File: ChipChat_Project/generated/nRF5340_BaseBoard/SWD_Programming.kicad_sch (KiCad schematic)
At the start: 1 part, among them J1 Connector_Generic:Conn_02x05_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

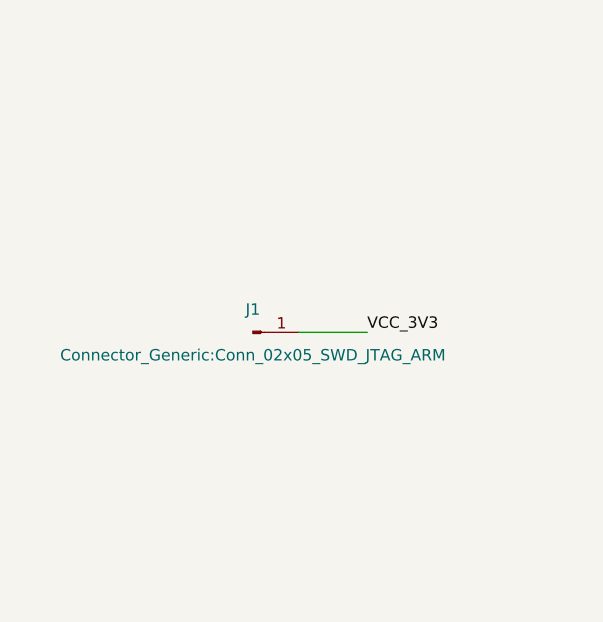
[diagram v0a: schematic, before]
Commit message: 💾 snapshot 2026-03-23_13-16-53
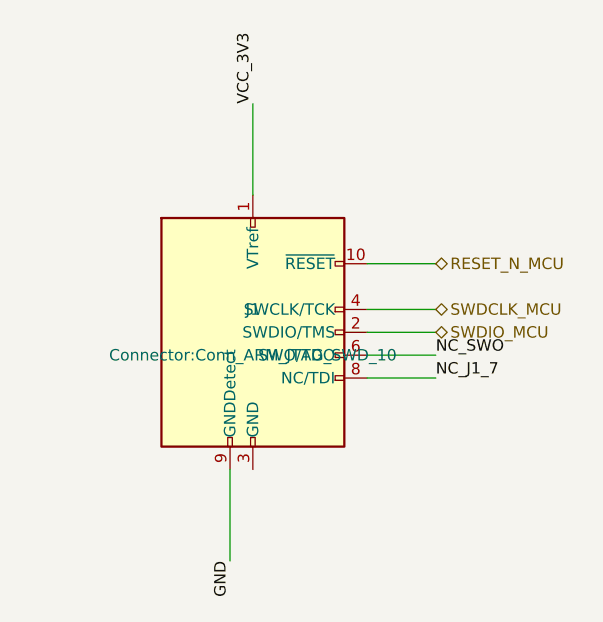
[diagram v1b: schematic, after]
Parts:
- removed J1: Connector_Generic:Conn_02x05_SWD_JTAG_ARM, symbol Conn_01x01_Pin
- added J1: Connector:Conn_ARM_JTAG_SWD_10, symbol Conn_ARM_JTAG_SWD_10
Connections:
- net VCC_3V3: now also J1.1 (VTref)
- new net: J1.3 (GND), J1.5 (GND)
- new net GND: J1.9 (GNDDetect)
- new net NC_J1_7: J1.8 (NC/TDI)
- new net NC_SWO: J1.6 (SWO/TDO)
- new net RESET_N_MCU: J1.10 (~{RESET})
- new net SWDCLK_MCU: J1.4 (SWCLK/TCK)
- new net SWDIO_MCU: J1.2 (SWDIO/TMS)
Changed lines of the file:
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@@
 	(paper "A4")
 	(symbol
-		(lib_id "Conn_01x01_Pin")
+		(lib_id "Conn_ARM_JTAG_SWD_10")
 		(at 200.0 100.0 0)
 		(unit 1)
@@
 			)
 		)
-		(property "Value" "Connector_Generic:Conn_02x05_SWD_JTAG_ARM"
+		(property "Value" "Connector:Conn_ARM_JTAG_SWD_10"
 			(at 200.0 102.54 0)
 			(effects
@@
 		(pin "1"
 		)
+		(pin "2"
+		)
+		(pin "3"
+		)
+		(pin "4"
+		)
+		(pin "5"
+		)
+		(pin "6"
+		)
+		(pin "7"
+		)
+		(pin "8"
+		)
+		(pin "9"
+		)
+		(pin "10"
+		)
 	)
 	(wire
 		(pts
-			(xy 205.08 100.0) (xy 212.7 100.0)
+			(xy 200.0 84.76) (xy 200.0 74.6)
 		)
 		(stroke
@@
 	)
 	(label "VCC_3V3"
-		(at 212.7 100.0 0)
+		(at 200.0 74.6 90)
 		(effects
 			(font
@@
 		)
 	)
+	(wire
+		(pts
+			(xy 212.7 100.0) (xy 220.32 100.0)
+		)
+		(stroke
+			(width 0)
+			(type default)
+		)
+	)
+	(hierarchical_label "SWDIO_MCU"
+		(shape bidirectional)
+		(at 220.32 100.0 0)
+		(effects
+			(font
+				(size 1.27 1.27)
+			)
+			(justify left)
+		)
+	)
+	(wire
+		(pts
+			(xy 197.46 115.24) (xy 197.46 125.4)
+		)
+		(stroke
+			(width 0)
+			(type default)
+		)
+	)
+	(label "GND"
+		(at 197.46 125.4 90)
+		(effects
+			(font
+				(size 1.27 1.27)
+			)
+			(justify right bottom)
+		)
+	)
+	(wire
+		(pts
+			(xy 212.7 97.46) (xy 220.32 97.46)
+		)
+		(stroke
+			(width 0)
+			(type default)
+		)
+	)
+	(hierarchical_label "SWDCLK_MCU"
+		(shape bidirectional)
+		(at 220.32 97.46 0)
+		(effects
+			(font
+				(size 1.27 1.27)
+			)
+			(justify left)
+		)
+	)
+	(wire
+		(pts
+			(xy 212.7 102.54) (xy 220.32 102.54)
+		)
+		(stroke
+			(width 0)
+			(type default)
+		)
+	)
+	(label "NC_SWO"
+		(at 220.32 102.54 0)
+		(effects
+			(font
+				(size 1.27 1.27)
+			)
+			(justify left bottom)
+		)
+	)
+	(wire
+		(pts
+			(xy 212.7 105.08) (xy 220.32 105.08)
+		)
+		(stroke
+			(width 0)
+			(type default)
+		)
+	)
+	(label "NC_J1_7"
+		(at 220.32 105.08 0)
+		(effects
+			(font
+				(size 1.27 1.27)
+			)
+			(justify left bottom)
+		)
+	)
+	(wire
+		(pts
+			(xy 212.7 92.38) (xy 220.32 92.38)
+		)
+		(stroke
+			(width 0)
+			(type default)
+		)
+	)
+	(hierarchical_label "RESET_N_MCU"
+		(shape bidirectional)
+		(at 220.32 92.38 0)
+		(effects
+			(font
+				(size 1.27 1.27)
+			)
+			(justify left)
+		)
+	)
